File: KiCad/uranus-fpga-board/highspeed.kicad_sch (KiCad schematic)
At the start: 7 parts, among them J1 ASP-134488-01, J2 TYPE-C-31-M-12, U6 FT232HL-REEL, U7 93LC56BT, U8 USBLC6-2SC6, U9 W25Q128JVSIQ, Y2 3225-12-20-10-10/4B

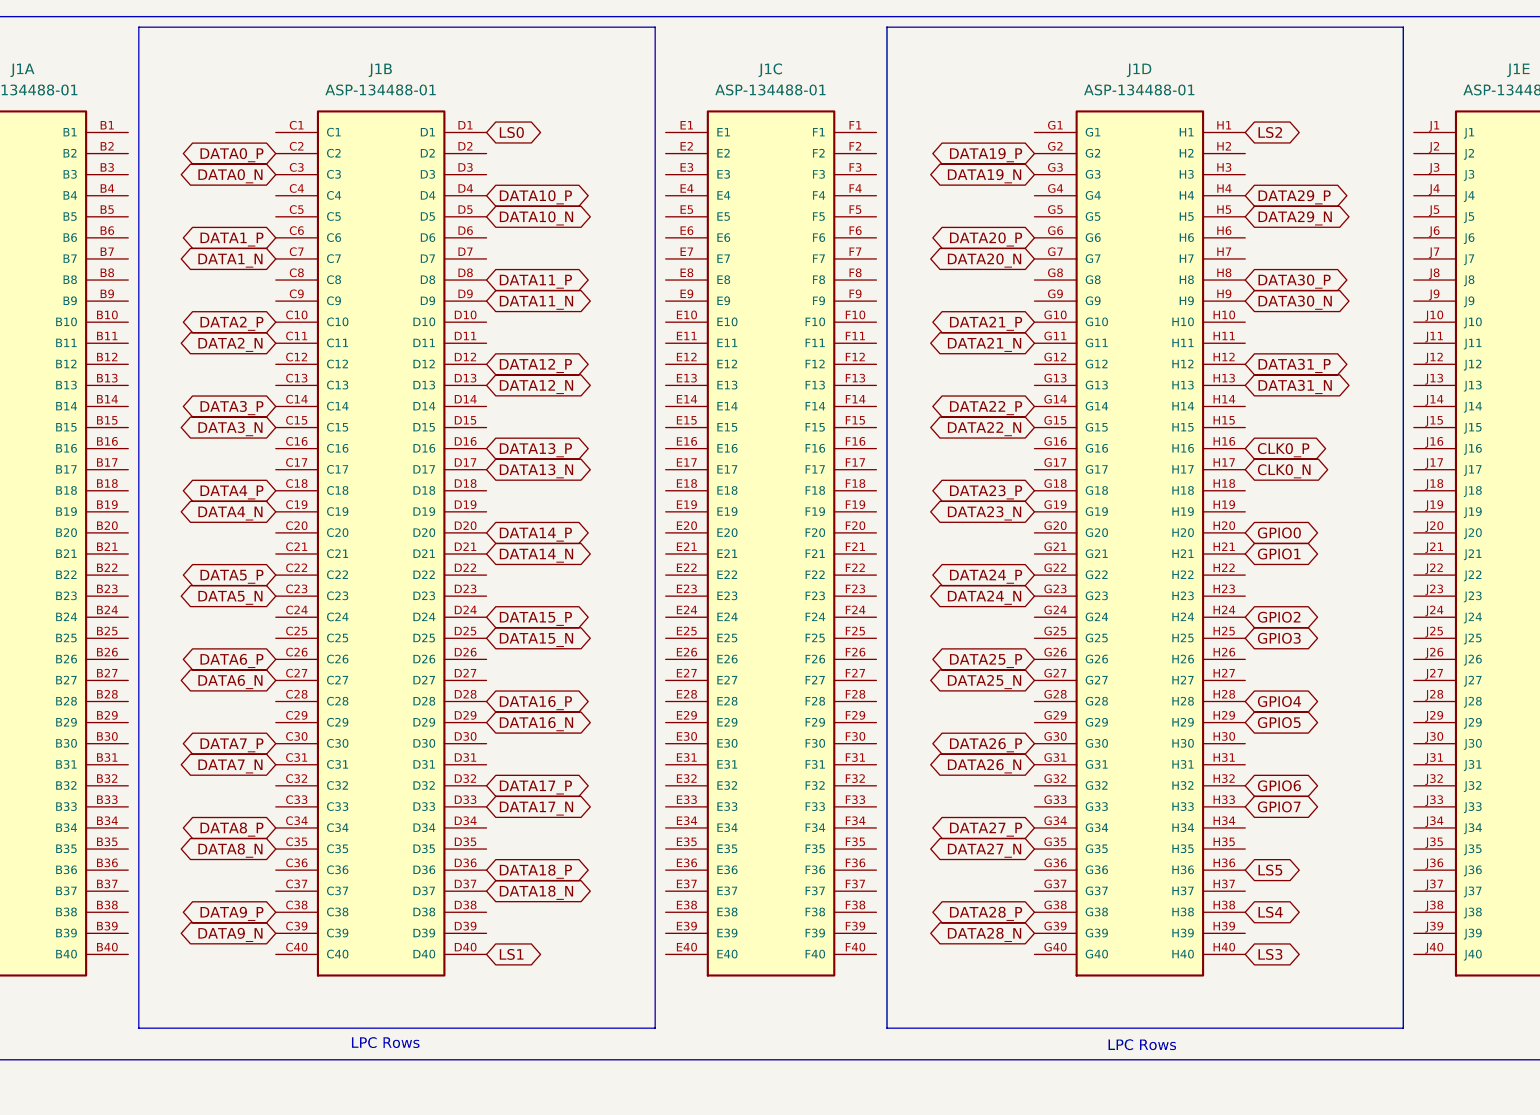
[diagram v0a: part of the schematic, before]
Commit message: New journal entry
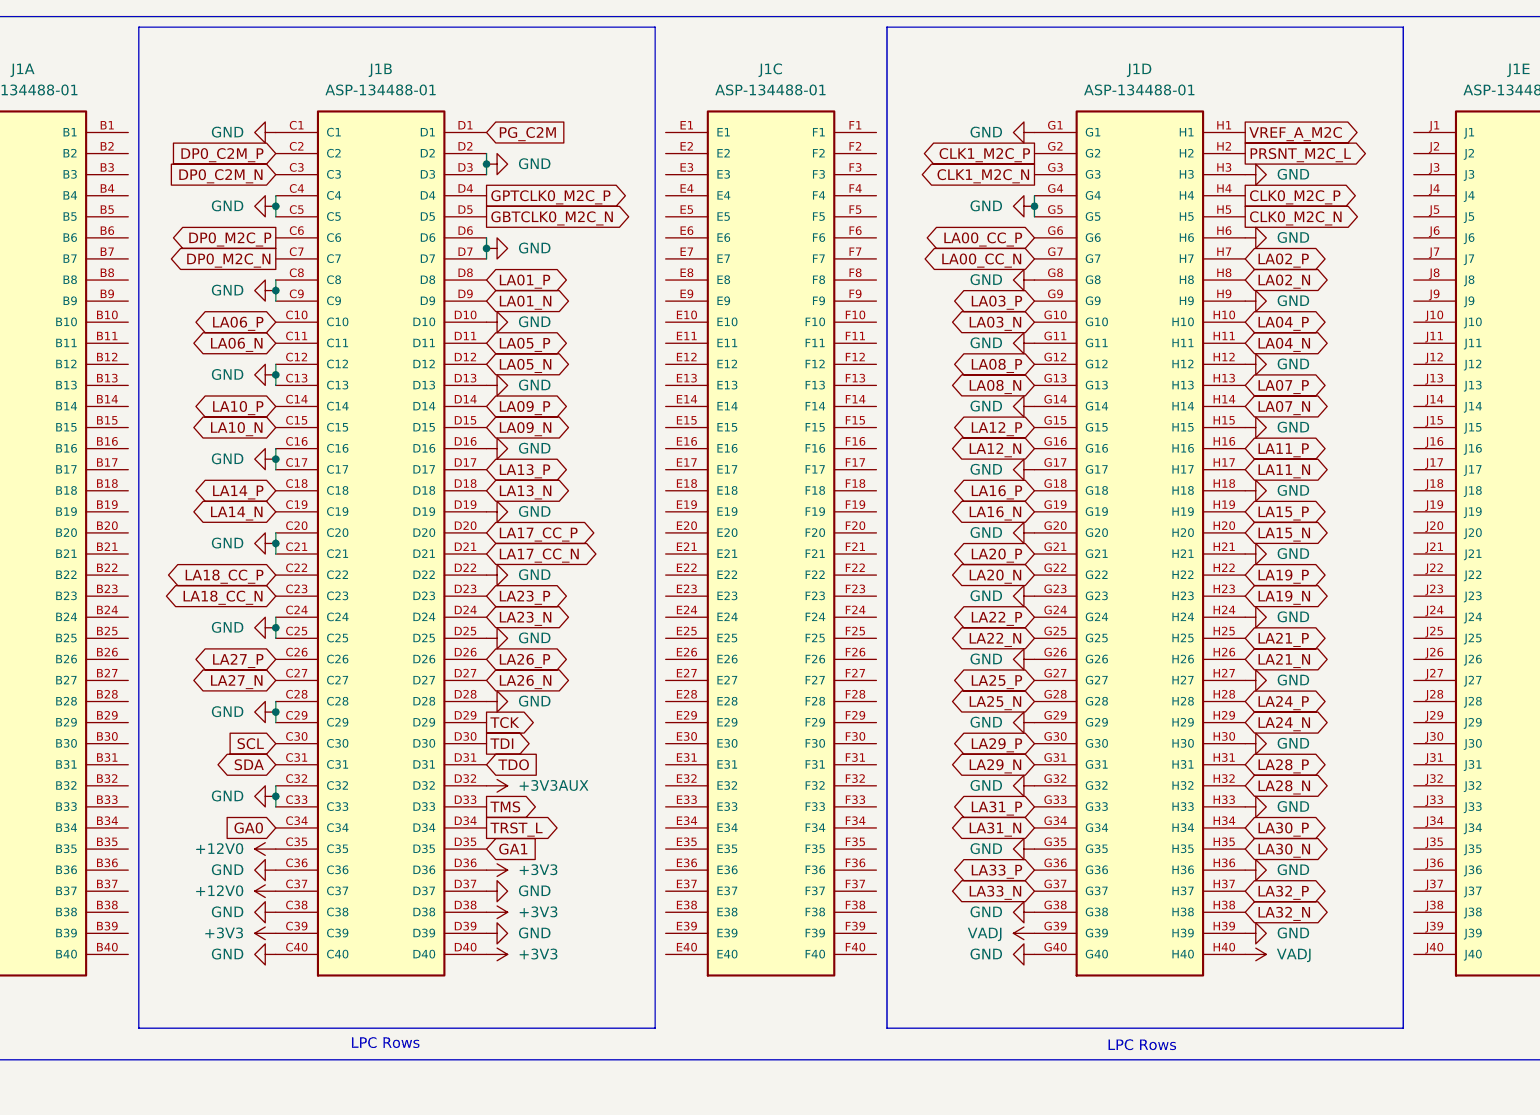
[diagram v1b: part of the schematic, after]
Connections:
- net DATA12_N is gone; now on net GND: J1.D13
- net DATA13_P is gone; now on net GND: J1.D16
- net DATA15_N is gone; now on net GND: J1.D25
- net DATA16_P is gone; now on net GND: J1.D28
- net DATA18_N is gone; now on net GND: J1.D37
- net DATA18_P is gone; now on net +3V3: J1.D36
- net DATA21_N is gone; now on net GND: J1.G11
- net DATA22_P is gone; now on net GND: J1.G14
- net DATA24_N is gone; now on net GND: J1.G23
- net DATA25_P is gone; now on net GND: J1.G26
- net DATA27_N is gone; now on net GND: J1.G35
- net DATA28_P is gone; now on net GND: J1.G38
- net DATA30_N is gone; now on net GND: J1.H9
- net DATA31_P is gone; now on net GND: J1.H12
- net DATA8_N is gone; now on net +12V0: J1.C35
- net DATA9_N is gone; now on net +3V3: J1.C39
- net DATA9_P is gone; now on net GND: J1.C38
- net GPIO1 is gone; now on net GND: J1.H21
- net GPIO2 is gone; now on net GND: J1.H24
- net GPIO7 is gone; now on net GND: J1.H33
- net LS1 is gone; now on net +3V3: J1.D40
- net LS3 is gone; now on net VADJ: J1.H40
- net LS5 is gone; now on net GND: J1.H36
- net GND: now also J1.C1, J1.C12, J1.C13, J1.C16, J1.C17, J1.C20, J1.C21, J1.C24, J1.C25, J1.C28, J1.C29, J1.C32, J1.C33, J1.C36, J1.C4, J1.C40, J1.C5, J1.C8, J1.C9, J1.D10, J1.D19, J1.D2, J1.D22, J1.D3, J1.D39, J1.D6, J1.D7, J1.G1, J1.G17, J1.G20, J1.G29, J1.G32, J1.G4, J1.G40, J1.G5, J1.G8, J1.H15, J1.H18, J1.H27, J1.H3, J1.H30, J1.H39, J1.H6
- net LA08_P: now reaches J1.G12
- net LA08_N: now reaches J1.G13
- net LA12_N: now reaches J1.G16
- net LA20_P: now reaches J1.G21
- net LA22_P: now reaches J1.G24
- net LA22_N: now reaches J1.G25
- net LA25_N: now reaches J1.G28
- net LA31_P: now reaches J1.G33
- net LA33_P: now reaches J1.G36
- net LA33_N: now reaches J1.G37
- net LA03_P: now reaches J1.G9
- net LA04_P: now reaches J1.H10
- net LA04_N: now reaches J1.H11
- net LA07_N: now reaches J1.H14
- net LA15_P: now reaches J1.H19
- net PRSNT_M2C_L: now reaches J1.H2
- net LA19_P: now reaches J1.H22
- net LA19_N: now reaches J1.H23
- net LA21_N: now reaches J1.H26
- net LA28_P: now reaches J1.H31
- net LA30_P: now reaches J1.H34
- net LA30_N: now reaches J1.H35
- net LA32_P: now reaches J1.H37
- net LA02_P: now reaches J1.H7
- net +12V0: now reaches J1.C37
- net LA05_P: now reaches J1.D11
- net LA09_P: now reaches J1.D14
- net LA09_N: now reaches J1.D15
- net LA13_N: now reaches J1.D18
- net LA23_P: now reaches J1.D23
- net LA26_P: now reaches J1.D26
- net LA26_N: now reaches J1.D27
- net TDI: now reaches J1.D30
- net TDO: now reaches J1.D31
- net TRST_L: now reaches J1.D34
- net GA1: now reaches J1.D35
- net +3V3: now reaches J1.D38
- net CLK0_N renamed LA11_N
- net CLK0_P renamed LA11_P
- net DATA0_N renamed DP0_C2M_N
- net DATA0_P renamed DP0_C2M_P
- net DATA10_N renamed GBTCLK0_M2C_N
- net DATA10_P renamed GPTCLK0_M2C_P
- net DATA11_N renamed LA01_N
- net DATA11_P renamed LA01_P
- net DATA12_P renamed LA05_N
- net DATA13_N renamed LA13_P
- net DATA14_N renamed LA17_CC_N
- net DATA14_P renamed LA17_CC_P
- net DATA15_P renamed LA23_N
- net DATA16_N renamed TCK
- net DATA17_N renamed TMS
- net DATA17_P renamed +3V3AUX
- net DATA19_N renamed CLK1_M2C_N
- net DATA19_P renamed CLK1_M2C_P
- net DATA1_N renamed DP0_M2C_N
- net DATA1_P renamed DP0_M2C_P
- net DATA20_N renamed LA00_CC_N
- net DATA20_P renamed LA00_CC_P
- net DATA21_P renamed LA03_N
- net DATA22_N renamed LA12_P
- net DATA23_N renamed LA16_N
- net DATA23_P renamed LA16_P
- net DATA24_P renamed LA20_N
- net DATA25_N renamed LA25_P
- net DATA26_N renamed LA29_N
- net DATA26_P renamed LA29_P
- net DATA27_P renamed LA31_N
- net DATA28_N renamed VADJ
- net DATA29_N renamed CLK0_M2C_N
- net DATA29_P renamed CLK0_M2C_P
- net DATA2_N renamed LA06_N
- net DATA2_P renamed LA06_P
- net DATA30_P renamed LA02_N
- net DATA31_N renamed LA07_P
- net DATA3_N renamed LA10_N
- net DATA3_P renamed LA10_P
- net DATA4_N renamed LA14_N
- net DATA4_P renamed LA14_P
- net DATA5_N renamed LA18_CC_N
- net DATA5_P renamed LA18_CC_P
- net DATA6_N renamed LA27_N
- net DATA6_P renamed LA27_P
- net DATA7_N renamed SDA
- net DATA7_P renamed SCL
- net DATA8_P renamed GA0
- net GPIO0 renamed LA15_N
- net GPIO3 renamed LA21_P
- net GPIO4 renamed LA24_P
- net GPIO5 renamed LA24_N
- net GPIO6 renamed LA28_N
- net LS0 renamed PG_C2M
- net LS2 renamed VREF_A_M2C
- net LS4 renamed LA32_N
